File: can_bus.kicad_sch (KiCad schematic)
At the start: 1 part, among them U8 MCP2562-E-SN

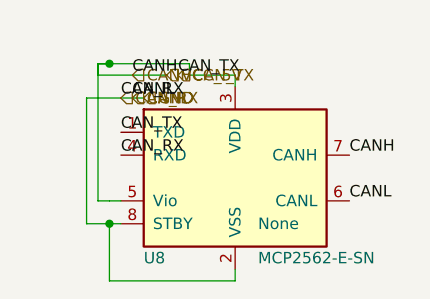
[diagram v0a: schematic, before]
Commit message: fic placer for small schemes
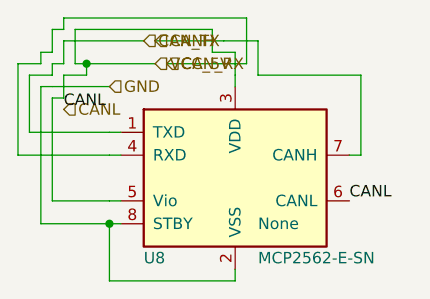
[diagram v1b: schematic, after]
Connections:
- net CANH: no longer U8.3 (VDD), U8.5 (Vio)
- net CANL: no longer U8.2 (VSS), U8.4 (RXD), U8.8 (STBY)
- new net CAN_RX: U8.4 (RXD)
- new net GND: U8.2 (VSS), U8.8 (STBY)
- new net VCC_5V: U8.3 (VDD), U8.5 (Vio)
